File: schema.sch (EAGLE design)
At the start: 19 parts, among them IC1 RT9011-CMGJ6, IC2 SX1308, J1 FH12-24S-0.5SH(55), U1 ESP-32S, X2 C-GRID-02-70543

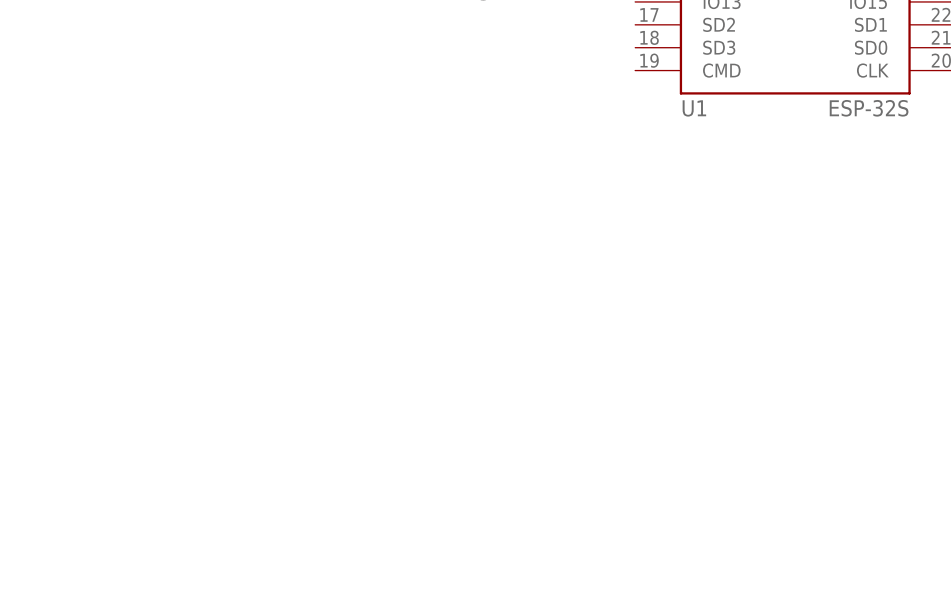
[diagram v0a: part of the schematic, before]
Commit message: Added new components
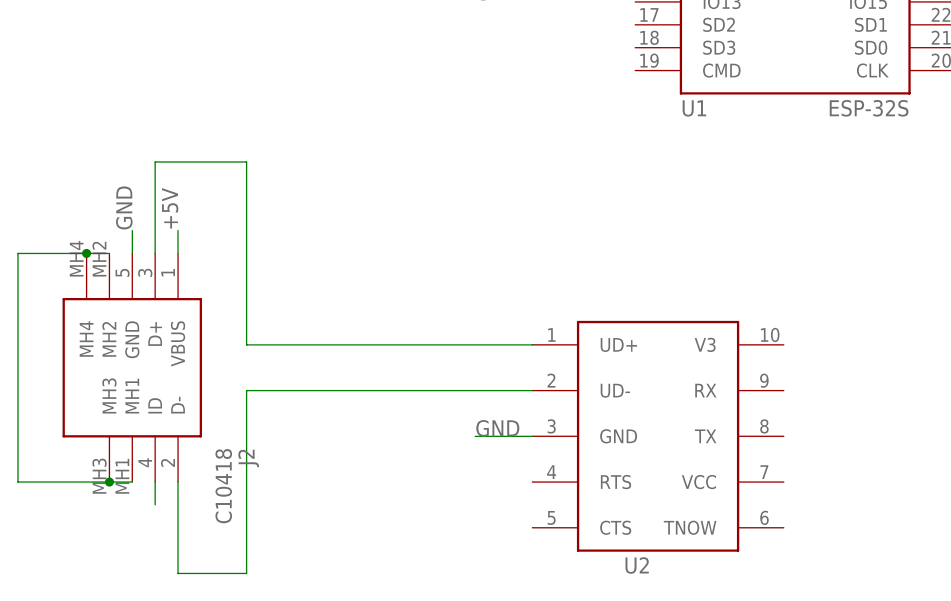
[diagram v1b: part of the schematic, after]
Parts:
- added J2: C10418, water-lib:C10418
- added U2: CH340ESMD, water-lib:CH340ESMD
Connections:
- new net D+: J2.D+, U2.UD+
- new net D-: J2.D-, U2.UD-
- new net N$10: J2.ID
- new net N$11: J2.MH1, J2.MH2, J2.MH3, J2.MH4
- net +5V: now also J2.VBUS
- net GND: now also J2.GND, U2.GND
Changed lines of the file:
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@@
 <?xml version="1.0" encoding="utf-8"?>
 <!DOCTYPE eagle SYSTEM "eagle.dtd">
-<eagle version="9.4.2">
+<eagle version="9.5.0">
 <drawing>
 <settings>
@@
 <part name="GND10" library="supply1" library_urn="urn:adsk.eagle:library:371" deviceset="GND" device=""/>
 <part name="C6" library="rcl" library_urn="urn:adsk.eagle:library:334" deviceset="C-EU" device="C0805" package3d_urn="urn:adsk.eagle:package:23617/2" value="22uF"/>
+<part name="U2" library="water-lib" deviceset="CH340E" device="SMD" package3d_urn="urn:adsk.eagle:package:3661278/1"/>
+<part name="J2" library="water-lib" deviceset="C10418" device=""/>
 </parts>
 <sheets>
@@
 <attribute name="NAME" x="49.784" y="180.721" size="1.778" layer="95"/>
 <attribute name="VALUE" x="49.784" y="175.641" size="1.778" layer="96"/>
+</instance>
+<instance part="U2" gate="G$1" x="-22.86" y="40.64" smashed="yes">
+<attribute name="NAME" x="-26.67" y="25.4" size="1.778" layer="95"/>
+</instance>
+<instance part="J2" gate="G$1" x="-76.2" y="60.96" smashed="yes" rot="R270">
+<attribute name="NAME" x="-68.58" y="39.37" size="1.778" layer="95" rot="R270" align="center-left"/>
+<attribute name="VALUE" x="-71.12" y="39.37" size="1.778" layer="96" rot="R270" align="center-left"/>
 </instance>
 </instances>
@@
 <junction x="55.88" y="162.56"/>
 </segment>
+<segment>
+<pinref part="U2" gate="G$1" pin="GND"/>
+<wire x1="-36.83" y1="40.64" x2="-43.18" y2="40.64" width="0.1524" layer="91"/>
+<label x="-43.18" y="40.64" size="1.778" layer="95"/>
+</segment>
+<segment>
+<pinref part="J2" gate="G$1" pin="GND"/>
+<wire x1="-81.28" y1="60.96" x2="-81.28" y2="63.5" width="0.1524" layer="91"/>
+<label x="-81.28" y="63.5" size="1.778" layer="95" rot="R90"/>
+</segment>
 </net>
 <net name="N$1" class="0">
@@
 <label x="43.18" y="193.04" size="1.778" layer="95" rot="R180" xref="yes"/>
 </segment>
-</net>
+<segment>
+<pinref part="J2" gate="G$1" pin="VBUS"/>
+<wire x1="-76.2" y1="60.96" x2="-76.2" y2="63.5" width="0.1524" layer="91"/>
+<label x="-76.2" y="63.5" size="1.778" layer="95" rot="R90"/>
+</segment>
+</net>
+<net name="D+" class="0">
+<segment>
+<pinref part="U2" gate="G$1" pin="UD+"/>
+<wire x1="-36.83" y1="50.8" x2="-68.58" y2="50.8" width="0.1524" layer="91"/>
+<wire x1="-68.58" y1="50.8" x2="-68.58" y2="71.12" width="0.1524" layer="91"/>
+<wire x1="-68.58" y1="71.12" x2="-78.74" y2="71.12" width="0.1524" layer="91"/>
+<pinref part="J2" gate="G$1" pin="D+"/>
+<wire x1="-78.74" y1="71.12" x2="-78.74" y2="60.96" width="0.1524" layer="91"/>
+</segment>
+</net>
+<net name="D-" class="0">
+<segment>
+<pinref part="U2" gate="G$1" pin="UD-"/>
+<wire x1="-36.83" y1="45.72" x2="-68.58" y2="45.72" width="0.1524" layer="91"/>
+<wire x1="-68.58" y1="45.72" x2="-68.58" y2="25.4" width="0.1524" layer="91"/>
+<wire x1="-68.58" y1="25.4" x2="-76.2" y2="25.4" width="0.1524" layer="91"/>
+<pinref part="J2" gate="G$1" pin="D-"/>
+<wire x1="-76.2" y1="25.4" x2="-76.2" y2="35.56" width="0.1524" layer="91"/>
+</segment>
+</net>
+<net name="N$10" class="0">
+<segment>
+<pinref part="J2" gate="G$1" pin="ID"/>
+<wire x1="-78.74" y1="35.56" x2="-78.74" y2="33.02" width="0.1524" layer="91"/>
+</segment>
+</net>
+<net name="N$11" class="0">
+<segment>
+<pinref part="J2" gate="G$1" pin="MH1"/>
+<pinref part="J2" gate="G$1" pin="MH3"/>
+<wire x1="-81.28" y1="35.56" x2="-83.82" y2="35.56" width="0.1524" layer="91"/>
+<wire x1="-83.82" y1="35.56" x2="-93.98" y2="35.56" width="0.1524" layer="91"/>
+<junction x="-83.82" y="35.56"/>
+<pinref part="J2" gate="G$1" pin="MH4"/>
+<wire x1="-93.98" y1="35.56" x2="-93.98" y2="60.96" width="0.1524" layer="91"/>
+<wire x1="-93.98" y1="60.96" x2="-86.36" y2="60.96" width="0.1524" layer="91"/>
+<pinref part="J2" gate="G$1" pin="MH2"/>
+<wire x1="-86.36" y1="60.96" x2="-83.82" y2="60.96" width="0.1524" layer="91"/>
+<junction x="-86.36" y="60.96"/>
+</segment>
+</net>
